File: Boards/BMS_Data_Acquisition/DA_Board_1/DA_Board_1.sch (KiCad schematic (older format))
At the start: 75 parts, among them J1 MM_M_VT_10, J2 MM_M_VT_12, J3 MM_M_VT_12, J4 MM_M_VT_12, J5 MM_M_VT_16, J6 MM_M_VT_12, J7 MM_M_VT_12, J8 MM_M_VT_10, J9 MM_M_VT_12, Q10 BSS308PE, Q12 BSS308PE, Q14 BSS308PE, Q16 BSS308PE, Q2 BSS308PE, Q4 BSS308PE, Q6 BSS308PE, Q8 BSS308PE, T0 Tab_Connect_BMS, T10 Tab_Connect_BMS, T12 Tab_Connect_BMS, T14 Tab_Connect_BMS, T16 Tab_Connect_BMS, T2 Tab_Connect_BMS, T4 Tab_Connect_BMS, T6 Tab_Connect_BMS, T8 Tab_Connect_BMS

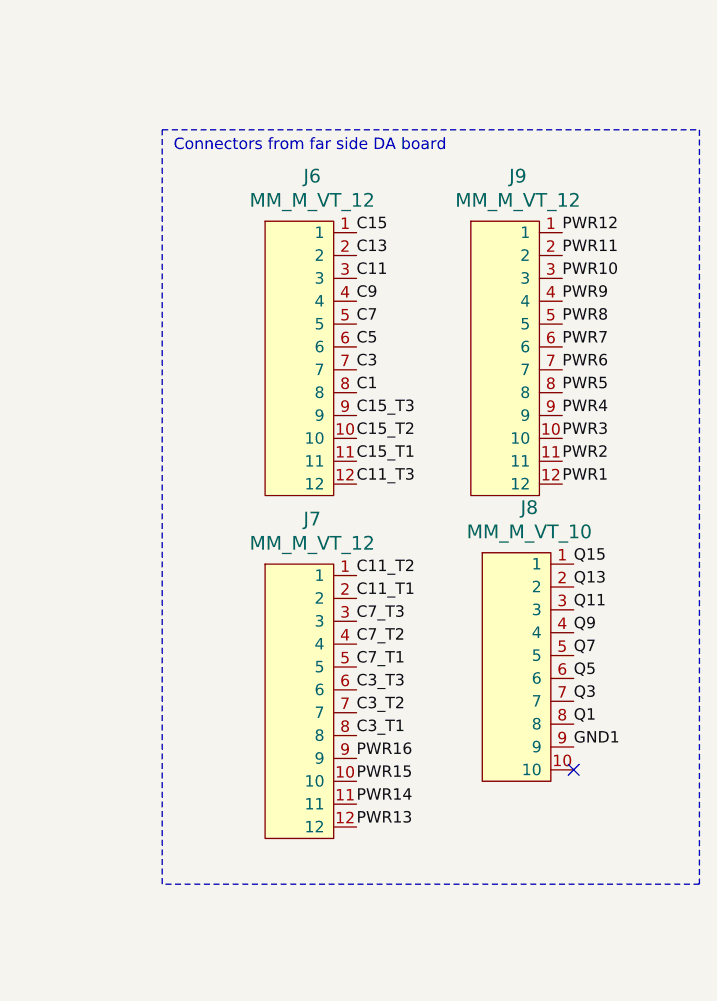
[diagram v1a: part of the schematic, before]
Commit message: Changes to DA_Board_1 Layout
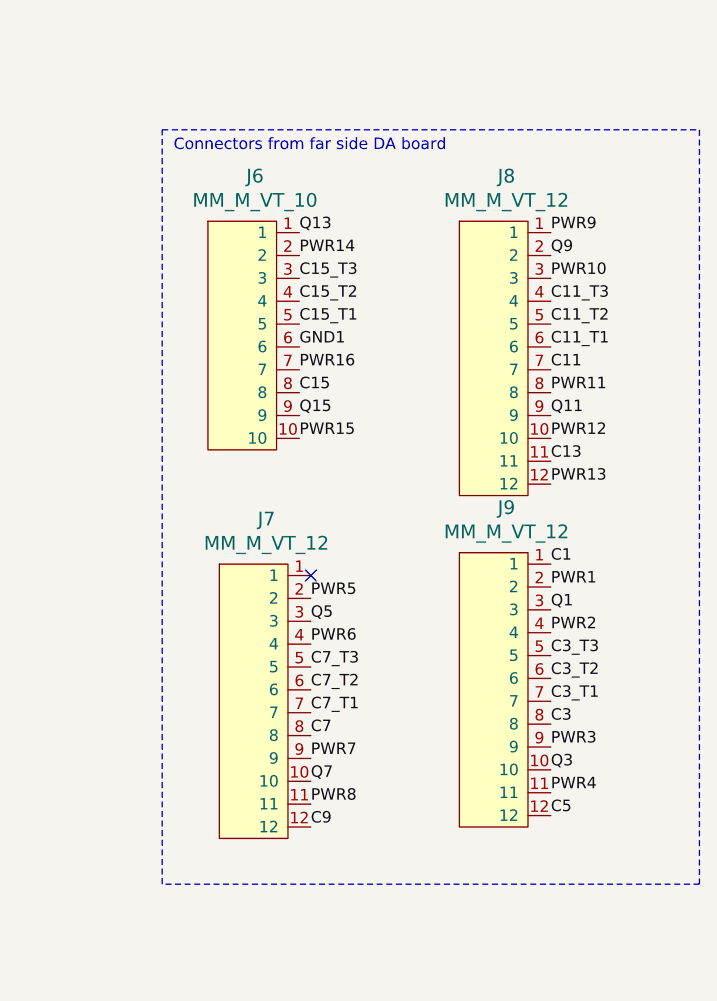
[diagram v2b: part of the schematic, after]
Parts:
- removed J6: MM_M_VT_12, footprints:micromatch_female_vert_12, symbol formula:MM_M_VT_12
- removed J8: MM_M_VT_10, footprints:micromatch_female_vert_10, symbol formula:MM_M_VT_10
- added J6: MM_M_VT_10, footprints:micromatch_female_vert_10, symbol formula:MM_M_VT_10
- added J8: MM_M_VT_12, footprints:micromatch_female_vert_12, symbol formula:MM_M_VT_12
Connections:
- net C1: now also J9.1
- net C11: now also J8.7
- net C11_T1: now also J8.6; no longer J7.2
- net C11_T2: now also J8.5; no longer J7.1
- net C11_T3: now also J8.4
- net C13: now also J8.11
- net C15: now also J6.8
- net C15_T1: now also J6.5
- net C15_T2: now also J6.4
- net C15_T3: now also J6.3
- net C3: now also J9.8
- net C3_T1: now also J9.7; no longer J7.8
- net C3_T2: now also J9.6; no longer J7.7
- net C3_T3: now also J9.5; no longer J7.6
- net C5: now also J9.12
- net C7: now also J7.8
- net C7_T1: now also J7.7; no longer J7.5
- net C7_T2: now also J7.6; no longer J7.4
- net C7_T3: now also J7.5; no longer J7.3
- net C9: now also J7.12
- net GND1: now also J6.6
- net PWR1: now also J9.2; no longer J9.12
- net PWR10: now also J8.3; no longer J9.3
- net PWR11: now also J8.8; no longer J9.2
- net PWR12: now also J8.10; no longer J9.1
- net PWR13: now also J8.12; no longer J7.12
- net PWR14: now also J6.2; no longer J7.11
- net PWR15: now also J6.10; no longer J7.10
- net PWR16: now also J6.7; no longer J7.9
- net PWR2: now also J9.4; no longer J9.11
- net PWR3: now also J9.9; no longer J9.10
- net PWR4: now also J9.11; no longer J9.9
- net PWR5: now also J7.2; no longer J9.8
- net PWR6: now also J7.4; no longer J9.7
- net PWR7: now also J7.9; no longer J9.6
- net PWR8: now also J7.11; no longer J9.5
- net PWR9: now also J8.1; no longer J9.4
- net Q1: now also J9.3
- net Q11: now also J8.9
- net Q13: now also J6.1
- net Q15: now also J6.9
- net Q3: now also J9.10
- net Q5: now also J7.3
- net Q7: now also J7.10
- net Q9: now also J8.2
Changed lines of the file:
@@
 EESchema Schematic File Version 4
 LIBS:DA_Board_1-cache
+LIBS:DA_Board_2-cache
 EELAYER 26 0
 EELAYER END
@@
 	3200 2200 3200 2350
 Connection ~ 3200 2200
-$Comp
-L formula:MM_M_VT_12 J6
-U 1 1 5E4EE95D
-P 9050 10950
-F 0 "J6" H 9006 12297 60  0000 C CNN
-F 1 "MM_M_VT_12" H 9006 12191 60  0000 C CNN
-F 2 "footprints:micromatch_female_vert_12" H 8850 12050 60  0001 C CNN
-F 3 "http://www.te.com/commerce/DocumentDelivery/DDEController?Action=showdoc&DocId=Customer+Drawing%7F338068%7FF1%7Fpdf%7FEnglish%7FENG_CD_338068_F1.pdf%7F1-1-215464-2" H 8950 12150 60  0001 C CNN
-F 4 "TE" H 9150 12350 60  0001 C CNN "MFN"
-F 5 "1-215464-2" H 9250 12450 60  0001 C CNN "MPN"
-F 6 "http://www.te.com/global-en/product-1-215464-2.html" H 9050 12250 60  0001 C CNN "PurchasingLink"
-	1    9050 10950
-	1    0    0    -1
-$EndComp
-$Comp
-L formula:MM_M_VT_12 J7
-U 1 1 5E4EE966
-P 9050 12450
-F 0 "J7" H 9006 13797 60  0000 C CNN
-F 1 "MM_M_VT_12" H 9006 13691 60  0000 C CNN
-F 2 "footprints:micromatch_female_vert_12" H 8850 13550 60  0001 C CNN
-F 3 "http://www.te.com/commerce/DocumentDelivery/DDEController?Action=showdoc&DocId=Customer+Drawing%7F338068%7FF1%7Fpdf%7FEnglish%7FENG_CD_338068_F1.pdf%7F1-1-215464-2" H 8950 13650 60  0001 C CNN
-F 4 "TE" H 9150 13850 60  0001 C CNN "MFN"
-F 5 "1-215464-2" H 9250 13950 60  0001 C CNN "MPN"
-F 6 "http://www.te.com/global-en/product-1-215464-2.html" H 9050 13750 60  0001 C CNN "PurchasingLink"
-	1    9050 12450
-	1    0    0    -1
-$EndComp
-$Comp
-L formula:MM_M_VT_10 J8
-U 1 1 5E4EE96F
-P 9900 11950
-F 0 "J8" H 9956 12847 60  0000 C CNN
-F 1 "MM_M_VT_10" H 9956 12741 60  0000 C CNN
-F 2 "footprints:micromatch_female_vert_10" H 9800 12600 60  0001 C CNN
-F 3 "http://www.te.com/commerce/DocumentDelivery/DDEController?Action=showdoc&DocId=Customer+Drawing%7F338068%7FF1%7Fpdf%7FEnglish%7FENG_CD_338068_F1.pdf%7F1-1-215464-0" H 9800 13150 60  0001 C CNN
-F 4 "TE" H 10000 13350 60  0001 C CNN "MFN"
-F 5 "1-215464-0" H 10100 13450 60  0001 C CNN "MPN"
-F 6 "http://www.te.com/global-en/product-1-215464-0.html" H 9900 13250 60  0001 C CNN "PurchasingLink"
-	1    9900 11950
-	1    0    0    -1
-$EndComp
-Text Label 9200 9850 0    50   ~ 0
-C15
-Text Label 9200 9950 0    50   ~ 0
-C13
-Text Label 9200 10050 0    50   ~ 0
-C11
-Text Label 9200 10150 0    50   ~ 0
-C9
-Text Label 9200 10250 0    50   ~ 0
-C7
-Text Label 9200 10350 0    50   ~ 0
-C5
-Text Label 9200 10450 0    50   ~ 0
-C3
-Text Label 9200 10550 0    50   ~ 0
-C1
-Text Label 9200 10650 0    50   ~ 0
-C15_T3
-Text Label 9200 10750 0    50   ~ 0
-C15_T2
-Text Label 9200 10850 0    50   ~ 0
-C15_T1
-Text Label 9200 10950 0    50   ~ 0
-C11_T3
-Text Label 9200 11350 0    50   ~ 0
-C11_T2
-Text Label 9200 11450 0    50   ~ 0
-C11_T1
-Text Label 9200 11550 0    50   ~ 0
-C7_T3
-Text Label 9200 11650 0    50   ~ 0
-C7_T2
-Text Label 9200 11750 0    50   ~ 0
-C7_T1
-Text Label 9200 11850 0    50   ~ 0
-C3_T3
-Text Label 9200 11950 0    50   ~ 0
-C3_T2
-Text Label 9200 12050 0    50   ~ 0
-C3_T1
-Text Label 9200 12350 0    50   ~ 0
-PWR14
-Text Label 9200 12450 0    50   ~ 0
-PWR13
-Text Label 10100 9850 0    50   ~ 0
-PWR12
-Text Label 10100 9950 0    50   ~ 0
-PWR11
-Text Label 10100 10050 0    50   ~ 0
-PWR10
-Text Label 10100 10150 0    50   ~ 0
-PWR9
-Text Label 10100 10250 0    50   ~ 0
-PWR8
-Text Label 10100 10350 0    50   ~ 0
-PWR7
-Text Label 10100 10450 0    50   ~ 0
-PWR6
-Text Label 10100 10550 0    50   ~ 0
-PWR5
-Text Label 10100 10650 0    50   ~ 0
-PWR4
-Text Label 10100 10750 0    50   ~ 0
-PWR3
-Text Label 10100 10850 0    50   ~ 0
-PWR2
-Text Label 10100 10950 0    50   ~ 0
-PWR1
-Text Label 10150 11300 0    50   ~ 0
-Q15
-Text Label 10150 11400 0    50   ~ 0
-Q13
-Text Label 10150 11500 0    50   ~ 0
-Q11
-Text Label 10150 11600 0    50   ~ 0
-Q9
-Text Label 10150 11700 0    50   ~ 0
-Q7
-Text Label 10150 11800 0    50   ~ 0
-Q5
-Text Label 10150 11900 0    50   ~ 0
-Q3
-Text Label 10150 12000 0    50   ~ 0
-Q1
-Text Label 10150 12100 0    50   ~ 0
-GND1
-Text Label 9200 12150 0    50   ~ 0
-PWR16
-Text Label 9200 12250 0    50   ~ 0
-PWR15
-$Comp
-L formula:MM_M_VT_12 J9
-U 1 1 5E4EE9A5
-P 9950 10950
-F 0 "J9" H 9906 12297 60  0000 C CNN
-F 1 "MM_M_VT_12" H 9906 12191 60  0000 C CNN
-F 2 "footprints:micromatch_female_vert_12" H 9750 12050 60  0001 C CNN
-F 3 "http://www.te.com/commerce/DocumentDelivery/DDEController?Action=showdoc&DocId=Customer+Drawing%7F338068%7FF1%7Fpdf%7FEnglish%7FENG_CD_338068_F1.pdf%7F1-1-215464-2" H 9850 12150 60  0001 C CNN
-F 4 "TE" H 10050 12350 60  0001 C CNN "MFN"
-F 5 "1-215464-2" H 10150 12450 60  0001 C CNN "MPN"
-F 6 "http://www.te.com/global-en/product-1-215464-2.html" H 9950 12250 60  0001 C CNN "PurchasingLink"
-	1    9950 10950
-	1    0    0    -1
-$EndComp
-NoConn ~ 10150 12200
 Wire Notes Line
 	8350 9400 10700 9400
@@
 	1    0    0    -1
 $EndComp
+$Comp
+L formula:MM_M_VT_12 J8
+U 1 1 5DC0F961
+P 9900 10950
+F 0 "J8" H 9856 12297 60  0000 C CNN
+F 1 "MM_M_VT_12" H 9856 12191 60  0000 C CNN
+F 2 "footprints:micromatch_female_vert_12" H 9700 12050 60  0001 C CNN
+F 3 "http://www.te.com/commerce/DocumentDelivery/DDEController?Action=showdoc&DocId=Customer+Drawing%7F338068%7FF1%7Fpdf%7FEnglish%7FENG_CD_338068_F1.pdf%7F1-1-215464-2" H 9800 12150 60  0001 C CNN
+F 4 "TE" H 10000 12350 60  0001 C CNN "MFN"
+F 5 "1-215464-2" H 10100 12450 60  0001 C CNN "MPN"
+F 6 "http://www.te.com/global-en/product-1-215464-2.html" H 9900 12250 60  0001 C CNN "PurchasingLink"
+	1    9900 10950
+	1    0    0    -1
+$EndComp
+$Comp
+L formula:MM_M_VT_12 J7
+U 1 1 5DC0F96B
+P 8850 12450
+F 0 "J7" H 8806 13797 60  0000 C CNN
+F 1 "MM_M_VT_12" H 8806 13691 60  0000 C CNN
+F 2 "footprints:micromatch_female_vert_12" H 8650 13550 60  0001 C CNN
+F 3 "http://www.te.com/commerce/DocumentDelivery/DDEController?Action=showdoc&DocId=Customer+Drawing%7F338068%7FF1%7Fpdf%7FEnglish%7FENG_CD_338068_F1.pdf%7F1-1-215464-2" H 8750 13650 60  0001 C CNN
+F 4 "TE" H 8950 13850 60  0001 C CNN "MFN"
+F 5 "1-215464-2" H 9050 13950 60  0001 C CNN "MPN"
+F 6 "http://www.te.com/global-en/product-1-215464-2.html" H 8850 13750 60  0001 C CNN "PurchasingLink"
+	1    8850 12450
+	1    0    0    -1
+$EndComp
+$Comp
+L formula:MM_M_VT_10 J6
+U 1 1 5DC0F975
+P 8700 10500
+F 0 "J6" H 8756 11397 60  0000 C CNN
+F 1 "MM_M_VT_10" H 8756 11291 60  0000 C CNN
+F 2 "footprints:micromatch_female_vert_10" H 8600 11150 60  0001 C CNN
+F 3 "http://www.te.com/commerce/DocumentDelivery/DDEController?Action=showdoc&DocId=Customer+Drawing%7F338068%7FF1%7Fpdf%7FEnglish%7FENG_CD_338068_F1.pdf%7F1-1-215464-0" H 8600 11700 60  0001 C CNN
+F 4 "TE" H 8800 11900 60  0001 C CNN "MFN"
+F 5 "1-215464-0" H 8900 12000 60  0001 C CNN "MPN"
+F 6 "http://www.te.com/global-en/product-1-215464-0.html" H 8700 11800 60  0001 C CNN "PurchasingLink"
+	1    8700 10500
+	1    0    0    -1
+$EndComp
+Text Label 8950 10550 0    50   ~ 0
+C15
+Text Label 10050 10850 0    50   ~ 0
+C13
+Text Label 10050 10450 0    50   ~ 0
+C11
+Text Label 9000 12450 0    50   ~ 0
+C9
+Text Label 9000 12050 0    50   ~ 0
+C7
+Text Label 10050 12400 0    50   ~ 0
+C5
+Text Label 10050 12000 0    50   ~ 0
+C3
+Text Label 10050 11300 0    50   ~ 0
+C1
+Text Label 8950 10050 0    50   ~ 0
+C15_T3
+Text Label 8950 10150 0    50   ~ 0
+C15_T2
+Text Label 8950 10250 0    50   ~ 0
+C15_T1
+Text Label 10050 10150 0    50   ~ 0
+C11_T3
+Text Label 10050 10250 0    50   ~ 0
+C11_T2
+Text Label 10050 10350 0    50   ~ 0
+C11_T1
+Text Label 9000 11750 0    50   ~ 0
+C7_T3
+Text Label 9000 11850 0    50   ~ 0
+C7_T2
+Text Label 9000 11950 0    50   ~ 0
+C7_T1
+Text Label 10050 11700 0    50   ~ 0
+C3_T3
+Text Label 10050 11800 0    50   ~ 0
+C3_T2
+Text Label 10050 11900 0    50   ~ 0
+C3_T1
+Text Label 8950 9950 0    50   ~ 0
+PWR14
+Text Label 10050 10950 0    50   ~ 0
+PWR13
+Text Label 10050 10750 0    50   ~ 0
+PWR12
+Text Label 10050 10550 0    50   ~ 0
+PWR11
+Text Label 10050 10050 0    50   ~ 0
+PWR10
+Text Label 10050 9850 0    50   ~ 0
+PWR9
+Text Label 9000 12350 0    50   ~ 0
+PWR8
+Text Label 9000 12150 0    50   ~ 0
+PWR7
+Text Label 9000 11650 0    50   ~ 0
+PWR6
+Text Label 9000 11450 0    50   ~ 0
+PWR5
+Text Label 10050 12300 0    50   ~ 0
+PWR4
+Text Label 10050 12100 0    50   ~ 0
+PWR3
+Text Label 10050 11600 0    50   ~ 0
+PWR2
+Text Label 10050 11400 0    50   ~ 0
+PWR1
+Text Label 8950 10650 0    50   ~ 0
+Q15
+Text Label 8950 9850 0    50   ~ 0
+Q13
+Text Label 10050 10650 0    50   ~ 0
+Q11
+Text Label 10050 9950 0    50   ~ 0
+Q9
+Text Label 9000 12250 0    50   ~ 0
+Q7
+Text Label 9000 11550 0    50   ~ 0
+Q5
+Text Label 10050 12200 0    50   ~ 0
+Q3
+Text Label 10050 11500 0    50   ~ 0
+Q1
+Text Label 8950 10350 0    50   ~ 0
+GND1
+Text Label 8950 10450 0    50   ~ 0
+PWR16
+Text Label 8950 10750 0    50   ~ 0
+PWR15
+$Comp
+L formula:MM_M_VT_12 J9
+U 1 1 5DC0F9AC
+P 9900 12400
+F 0 "J9" H 9856 13747 60  0000 C CNN
+F 1 "MM_M_VT_12" H 9856 13641 60  0000 C CNN
+F 2 "footprints:micromatch_female_vert_12" H 9700 13500 60  0001 C CNN
+F 3 "http://www.te.com/commerce/DocumentDelivery/DDEController?Action=showdoc&DocId=Customer+Drawing%7F338068%7FF1%7Fpdf%7FEnglish%7FENG_CD_338068_F1.pdf%7F1-1-215464-2" H 9800 13600 60  0001 C CNN
+F 4 "TE" H 10000 13800 60  0001 C CNN "MFN"
+F 5 "1-215464-2" H 10100 13900 60  0001 C CNN "MPN"
+F 6 "http://www.te.com/global-en/product-1-215464-2.html" H 9900 13700 60  0001 C CNN "PurchasingLink"
+	1    9900 12400
+	1    0    0    -1
+$EndComp
+NoConn ~ 9000 11350
 $EndSCHEMATC
